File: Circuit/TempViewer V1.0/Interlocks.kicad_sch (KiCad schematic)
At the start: 32 parts, among them K1 EE2-5NU, K2 EE2-5NU, K3 EE2-5NU, K4 EE2-5NU, Q10 DMN3731U, Q3 DMN3731U, Q4 DMN3731U, Q5 DMN3731U, Q6 DMN3731U, Q7 DMN3731U, Q8 DMN3731U, Q9 DMN3731U

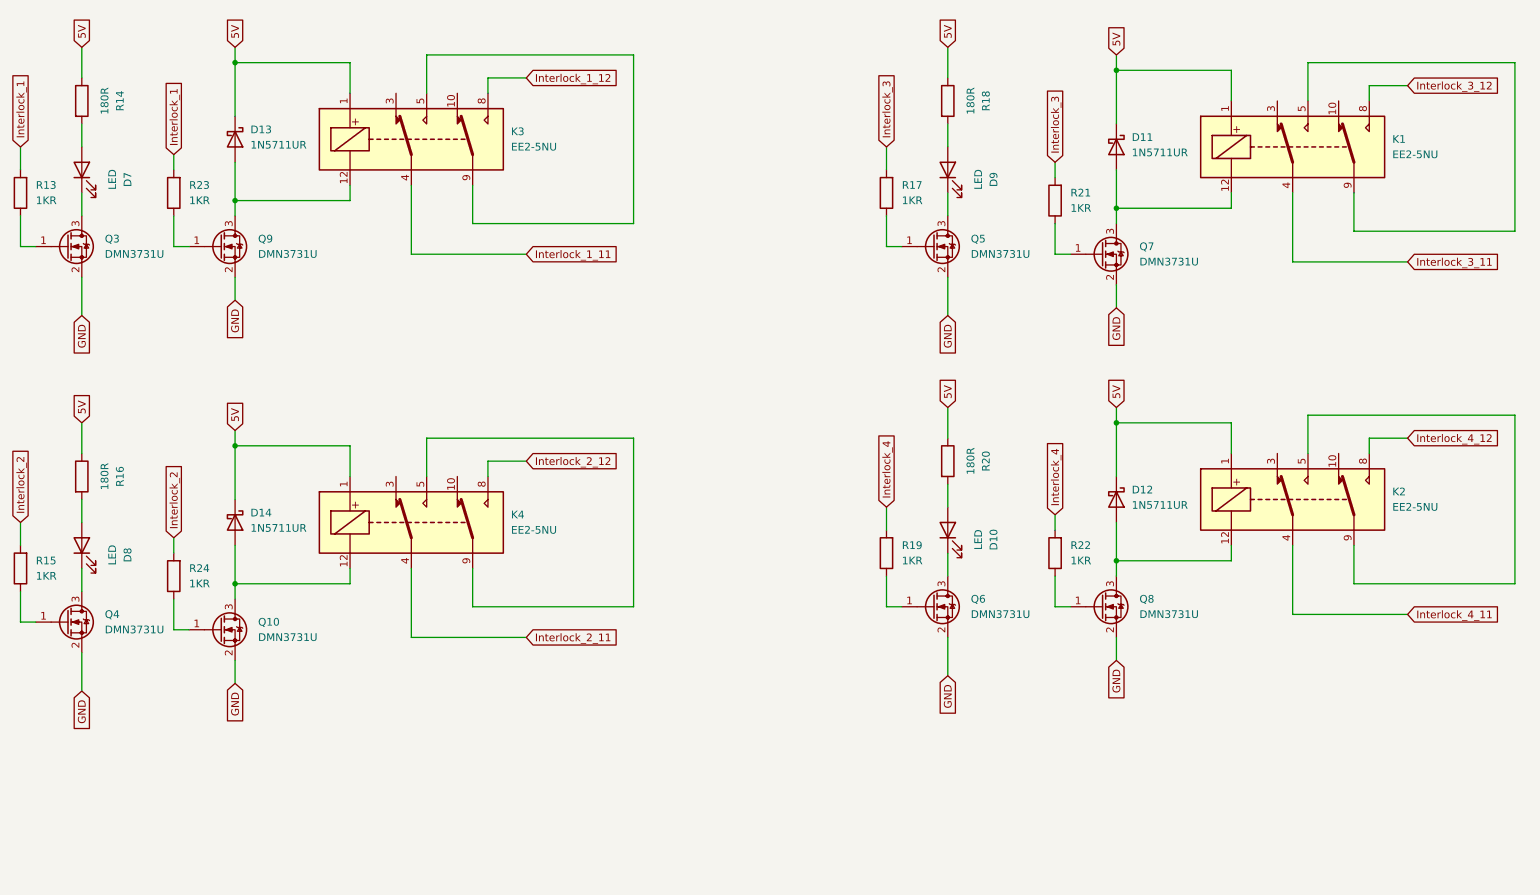
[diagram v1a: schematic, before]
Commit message: Update
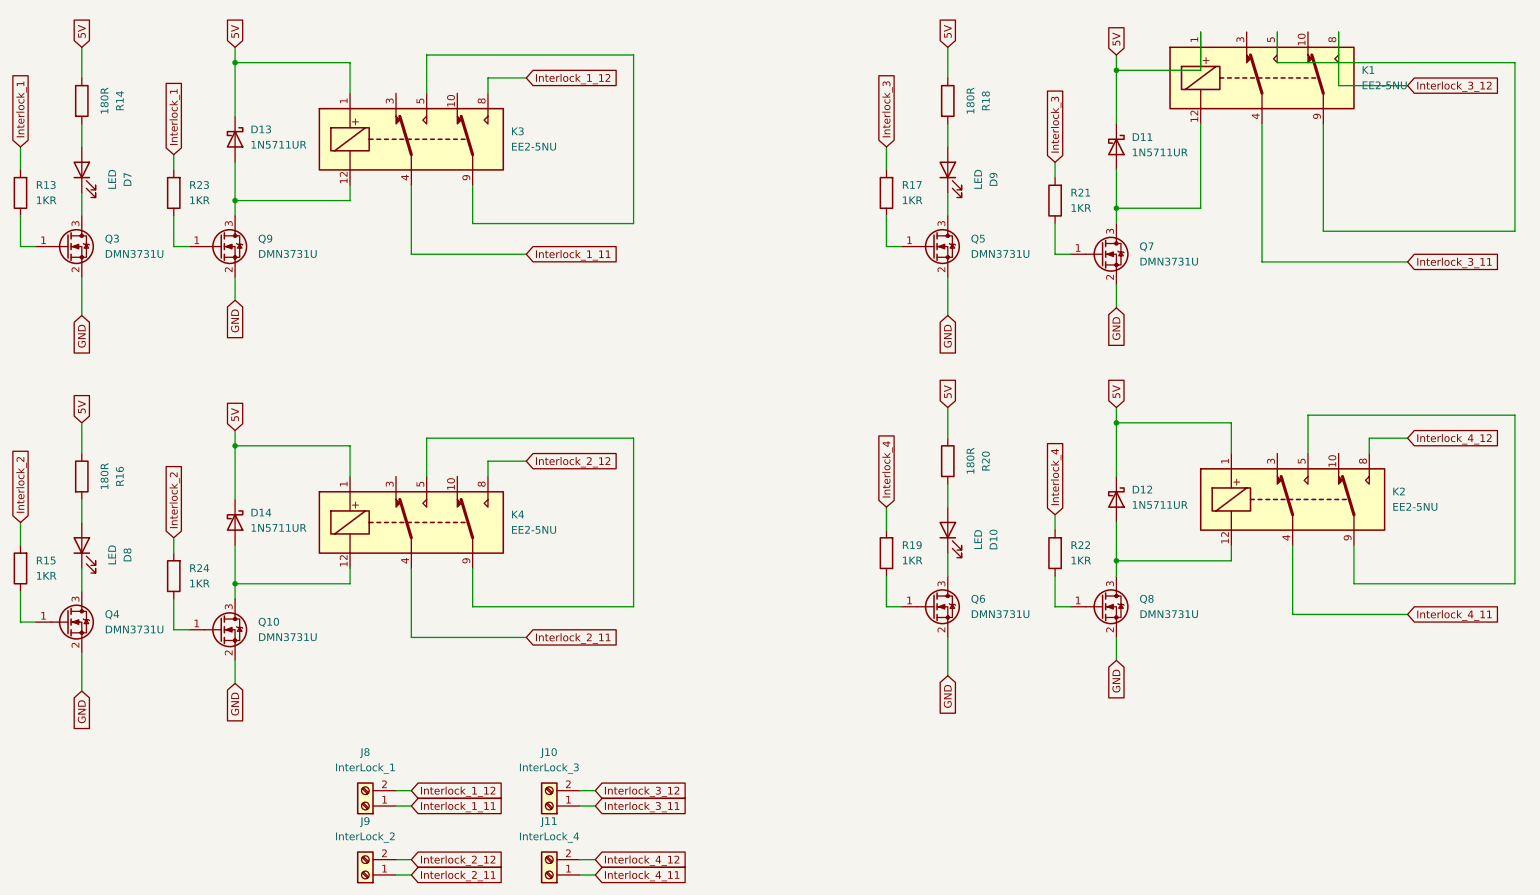
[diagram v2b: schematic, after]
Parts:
- added J10: InterLock_3, TerminalBlock_Phoenix:TerminalBlock_Phoenix_MKDS-3-2-5.08_1x02_P5.08mm_Horizontal, symbol Connector:Screw_Terminal_01x02
- added J11: InterLock_4, TerminalBlock_Phoenix:TerminalBlock_Phoenix_MKDS-3-2-5.08_1x02_P5.08mm_Horizontal, symbol Connector:Screw_Terminal_01x02
- added J8: InterLock_1, TerminalBlock_Phoenix:TerminalBlock_Phoenix_MKDS-3-2-5.08_1x02_P5.08mm_Horizontal, symbol Connector:Screw_Terminal_01x02
- added J9: InterLock_2, TerminalBlock_Phoenix:TerminalBlock_Phoenix_MKDS-3-2-5.08_1x02_P5.08mm_Horizontal, symbol Connector:Screw_Terminal_01x02
- K1, K2, K3, K4: footprint Relay_THT:Relay_SPST_Omron-G5Q-1A -> MY_SMD_LIB:EE2NU_KEM
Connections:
- net Interlock_1_11: now also J8.1 (Pin_1)
- net Interlock_1_12: now also J8.2 (Pin_2)
- net Interlock_2_11: now also J9.1 (Pin_1)
- net Interlock_2_12: now also J9.2 (Pin_2)
- net Interlock_3_11: now also J10.1 (Pin_1)
- net Interlock_3_12: now also J10.2 (Pin_2)
- net Interlock_4_11: now also J11.1 (Pin_1)
- net Interlock_4_12: now also J11.2 (Pin_2)
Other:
- moved on the sheet: K1
